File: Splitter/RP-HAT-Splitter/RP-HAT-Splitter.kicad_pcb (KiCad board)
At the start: 4 copper layers, 65 x 56 mm, 19 parts, among them J1 GPIO, J2 Conn_01x04_Socket, J3 Conn_01x04_Socket, J4 Conn_01x04_Socket, J5 Conn_01x04_Socket, J6 Conn_01x04_Socket, J7 Conn_01x04_Socket, U1 CAT24C256

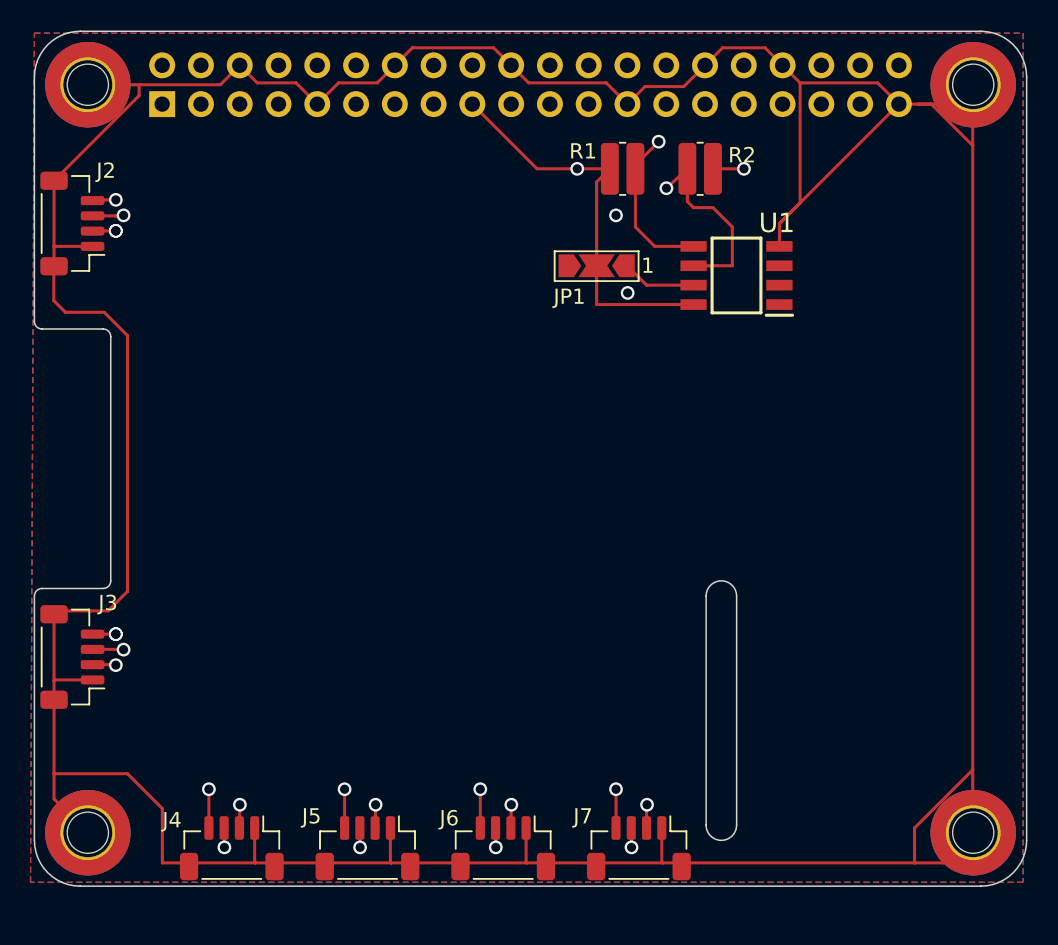
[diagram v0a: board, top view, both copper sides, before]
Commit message: asd
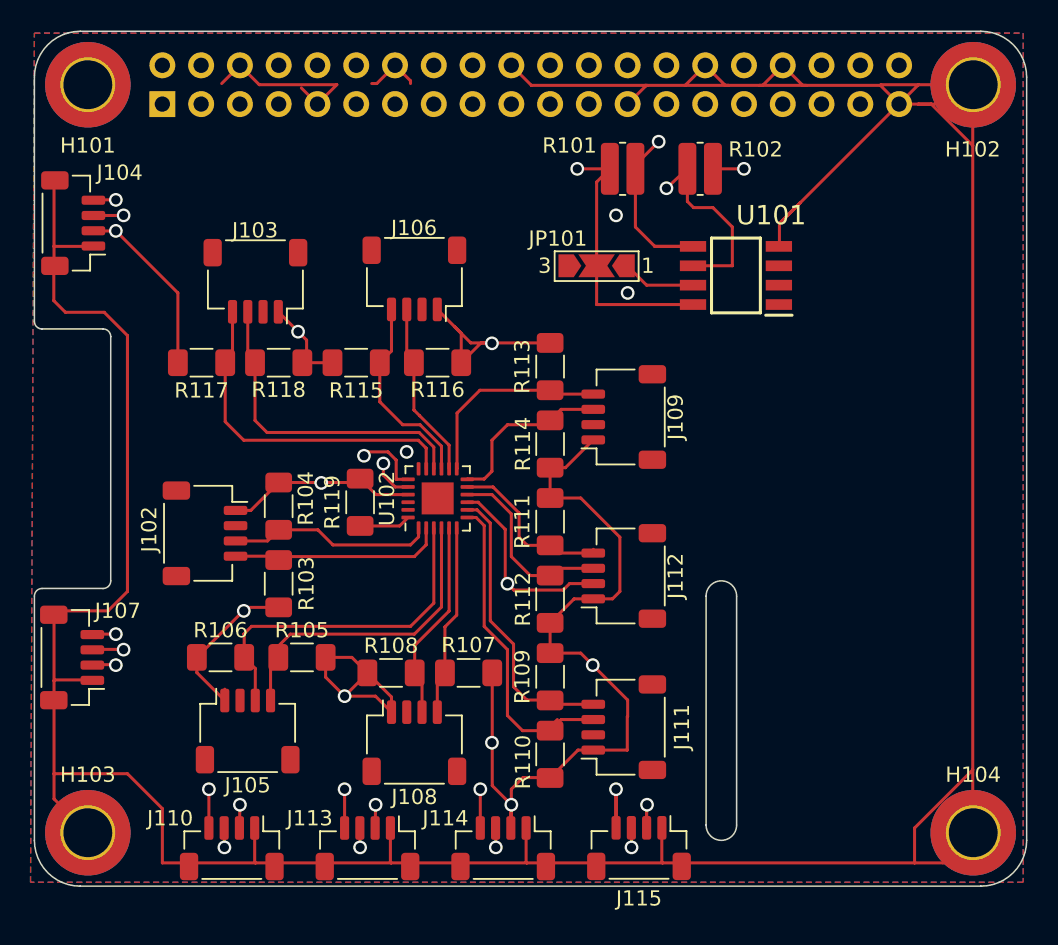
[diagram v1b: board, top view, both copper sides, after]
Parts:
- removed H1, H2, H3, H4: MountingHole_Pad, MountingHole:MountingHole_3.2mm_M3_DIN965_Pad_TopBottom
- removed J1: GPIO, Connector_PinSocket_2.54mm:PinSocket_2x20_P2.54mm_Vertical
- removed J2, J3, J4, J5, J6, J7: Conn_01x04_Socket, Connector_JST:JST_SH_BM04B-SRSS-TB_1x04-1MP_P1.00mm_Vertical
- removed JP1: ID_WP, Jumper:SolderJumper-3_P2.0mm_Open_TrianglePad1.0x1.5mm_NumberLabels
- removed MH1, MH2, MH3, MH4: MountingHole_2.7mm_M2.5, MountingHole:MountingHole_2.7mm_M2.5
- removed R1, R2: 3.9k, Resistor_SMD:R_0612_1632Metric_Pad1.18x3.40mm_HandSolder
- removed U1: CAT24C256, SamacSys:SOIC127P600X175-8M
- added H101: MountingHole_Pad, MountingHole:MountingHole_3.2mm_M3_DIN965_Pad_TopBottom, F.Cu at (103.5, 47.5)
- added H102: MountingHole_Pad, MountingHole:MountingHole_3.2mm_M3_DIN965_Pad_TopBottom, F.Cu at (161.5, 47.5)
- added H103: MountingHole_Pad, MountingHole:MountingHole_3.2mm_M3_DIN965_Pad_TopBottom, F.Cu at (103.5, 96.5)
- added H104: MountingHole_Pad, MountingHole:MountingHole_3.2mm_M3_DIN965_Pad_TopBottom, F.Cu at (161.5, 96.5)
- added J101: GPIO, Connector_PinSocket_2.54mm:PinSocket_2x20_P2.54mm_Vertical, B.Cu at (108.4, 48.8)
- added J102: I2C1-Multi0, Connector_JST:JST_SH_SM04B-SRSS-TB_1x04-1MP_P1.00mm_Horizontal, F.Cu at (111.2, 76.9)
- added J103: I2C1-Multi7, Connector_JST:JST_SH_SM04B-SRSS-TB_1x04-1MP_P1.00mm_Horizontal, F.Cu at (114.5, 60.4)
- added J104: I2C1-Normal, Connector_JST:JST_SH_BM04B-SRSS-TB_1x04-1MP_P1.00mm_Vertical, F.Cu at (102.5, 56.6)
- added J105: I2C1-Multi1, Connector_JST:JST_SH_SM04B-SRSS-TB_1x04-1MP_P1.00mm_Horizontal, F.Cu at (114.0, 89.8)
- added J106: I2C1-Multi6, Connector_JST:JST_SH_SM04B-SRSS-TB_1x04-1MP_P1.00mm_Horizontal, F.Cu at (124.9, 60.2)
- added J107: I2C1-Normal, Connector_JST:JST_SH_BM04B-SRSS-TB_1x04-1MP_P1.00mm_Vertical, F.Cu at (102.5, 85.0)
- added J108: I2C1-Multi2, Connector_JST:JST_SH_SM04B-SRSS-TB_1x04-1MP_P1.00mm_Horizontal, F.Cu at (124.9, 90.6)
- added J109: I2C1-Multi5, Connector_JST:JST_SH_SM04B-SRSS-TB_1x04-1MP_P1.00mm_Horizontal, F.Cu at (138.6, 69.3)
- added J110: I2C1-Normal, Connector_JST:JST_SH_BM04B-SRSS-TB_1x04-1MP_P1.00mm_Vertical, F.Cu at (112.9, 97.5)
- added J111: I2C1-Multi3, Connector_JST:JST_SH_SM04B-SRSS-TB_1x04-1MP_P1.00mm_Horizontal, F.Cu at (138.6, 89.6)
- added J112: I2C1-Multi4, Connector_JST:JST_SH_SM04B-SRSS-TB_1x04-1MP_P1.00mm_Horizontal, F.Cu at (138.6, 79.7)
- added J113: I2C1-Normal, Connector_JST:JST_SH_BM04B-SRSS-TB_1x04-1MP_P1.00mm_Vertical, F.Cu at (121.8, 97.5)
- added J114: I2C1-Normal, Connector_JST:JST_SH_BM04B-SRSS-TB_1x04-1MP_P1.00mm_Vertical, F.Cu at (130.7, 97.5)
- added J115: I2C1-Normal, Connector_JST:JST_SH_BM04B-SRSS-TB_1x04-1MP_P1.00mm_Vertical, F.Cu at (139.6, 97.5)
- added JP101: ID_WP, Jumper:SolderJumper-3_P2.0mm_Open_TrianglePad1.0x1.5mm_NumberLabels, F.Cu at (136.8, 59.4)
- added R101: 3.9k, Resistor_SMD:R_0612_1632Metric_Pad1.18x3.40mm_HandSolder, F.Cu at (138.5, 53.0)
- added R102: 3.9k, Resistor_SMD:R_0612_1632Metric_Pad1.18x3.40mm_HandSolder, F.Cu at (143.6, 53.0)
- added R103: 4k7, Resistor_SMD:R_1206_3216Metric_Pad1.30x1.75mm_HandSolder, F.Cu at (116.0, 80.2)
- added R104: 4k7, Resistor_SMD:R_1206_3216Metric_Pad1.30x1.75mm_HandSolder, F.Cu at (116.0, 75.1)
- added R105: 4k7, Resistor_SMD:R_1206_3216Metric_Pad1.30x1.75mm_HandSolder, F.Cu at (117.5, 85.0)
- added R106: 4k7, Resistor_SMD:R_1206_3216Metric_Pad1.30x1.75mm_HandSolder, F.Cu at (112.2, 85.0)
- added R107: 4k7, Resistor_SMD:R_1206_3216Metric_Pad1.30x1.75mm_HandSolder, F.Cu at (128.4, 86.0)
- added R108: 4k7, Resistor_SMD:R_1206_3216Metric_Pad1.30x1.75mm_HandSolder, F.Cu at (123.4, 86.0)
- added R109: 4k7, Resistor_SMD:R_1206_3216Metric_Pad1.30x1.75mm_HandSolder, F.Cu at (133.8, 86.3)
- added R110: 4k7, Resistor_SMD:R_1206_3216Metric_Pad1.30x1.75mm_HandSolder, F.Cu at (133.8, 91.4)
- added R111: 4k7, Resistor_SMD:R_1206_3216Metric_Pad1.30x1.75mm_HandSolder, F.Cu at (133.8, 76.1)
- added R112: 4k7, Resistor_SMD:R_1206_3216Metric_Pad1.30x1.75mm_HandSolder, F.Cu at (133.8, 81.2)
- added R113: 4k7, Resistor_SMD:R_1206_3216Metric_Pad1.30x1.75mm_HandSolder, F.Cu at (133.8, 66.0)
- added R114: 4k7, Resistor_SMD:R_1206_3216Metric_Pad1.30x1.75mm_HandSolder, F.Cu at (133.8, 71.0)
- added R115: 4k7, Resistor_SMD:R_1206_3216Metric_Pad1.30x1.75mm_HandSolder, F.Cu at (121.1, 65.7)
- added R116: 4k7, Resistor_SMD:R_1206_3216Metric_Pad1.30x1.75mm_HandSolder, F.Cu at (126.4, 65.7)
- added R117: 4k7, Resistor_SMD:R_1206_3216Metric_Pad1.30x1.75mm_HandSolder, F.Cu at (110.9, 65.7)
- added R118: 4k7, Resistor_SMD:R_1206_3216Metric_Pad1.30x1.75mm_HandSolder, F.Cu at (116.0, 65.7)
- added R119: 4k7, Resistor_SMD:R_1206_3216Metric_Pad1.30x1.75mm_HandSolder, F.Cu at (121.3, 74.9)
- added U101: CAT24C256, SamacSys:SOIC127P600X175-8M, F.Cu at (146.0, 60.0)
- added U102: PCA9548ARGE, Package_DFN_QFN:Texas_RGE0024C_EP2.1x2.1mm, F.Cu at (126.4, 74.6)
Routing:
- net +3V3: track 158.9 -> 254.5 mm, vias 9 -> 15
- net I2C1_SDA: track 107.7 -> 147.3 mm, vias 6 -> 7
- net I2C1_SCL: track 97.9 -> 131.7 mm
- net Net-(J105-Pin_3): track 0.00 -> 22.9 mm
- net Net-(J103-Pin_4): track 0.00 -> 22.6 mm
- net Net-(J111-Pin_3): track 0.00 -> 21.4 mm
- net Net-(J103-Pin_3): track 0.00 -> 21.3 mm
- net Net-(J105-Pin_4): track 0.00 -> 20.7 mm
- net Net-(J111-Pin_4): track 0.00 -> 18.9 mm
- net Net-(J102-Pin_4): track 0.00 -> 14.1 mm
- net Net-(J102-Pin_3): track 0.00 -> 13.5 mm
- net Net-(J109-Pin_4): track 0.00 -> 13.3 mm
- net Net-(J108-Pin_3): track 0.00 -> 13.2 mm
- net Net-(J106-Pin_4): track 0.00 -> 13.1 mm
- net Net-(J108-Pin_4): track 0.00 -> 12.6 mm
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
